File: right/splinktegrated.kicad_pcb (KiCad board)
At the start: 4 copper layers, 72.5 x 88.4 mm, 81 parts, among them J1 USB_C_Receptacle_USB2.0, J10 NA_Ribbon, J13 Conn_01x01_Socket, J14 Cirque, J15 Conn_01x01_Socket, J16 Conn_01x01_Socket, J17 Conn_01x01_Socket, J18 USB_C_Receptacle_USB2.0, J19 Conn_01x01_Socket, J20 Conn_01x01_Socket, J5 Conn_01x02, J6 Cirque, J7 NA_trackball, J8 NA_Ribbon, J9 NA_RGB, Q4 AO3401A, Q5 AO3401A, SW2 NA_SW_SPST, U1 RP2040, U2 USBLC6-2P6, U3 XC6210B332MR-G, U4 USBLC6-2P6, U5 W25Q128JVS, U6 74LVC1T45, Y1 Crystal_GND24

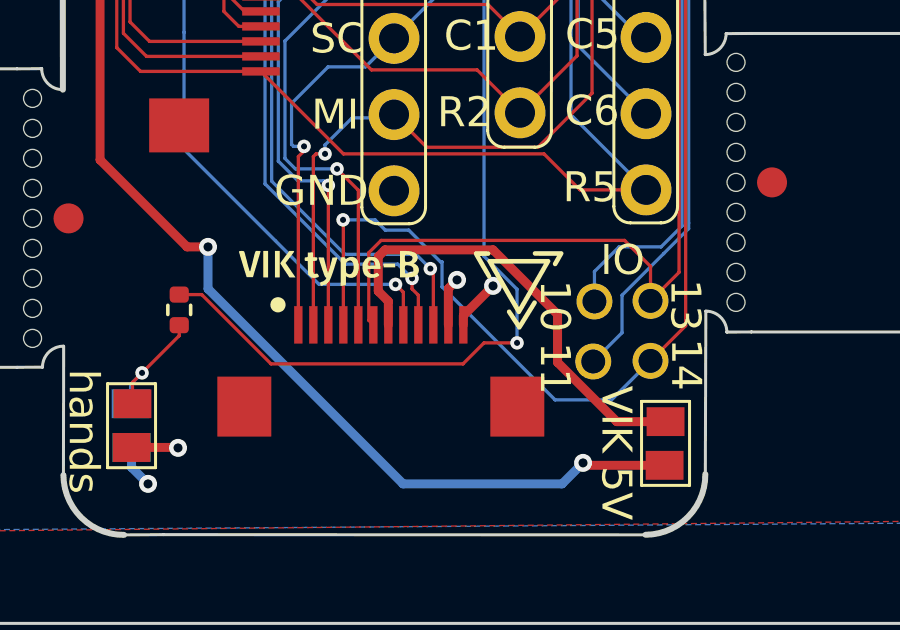
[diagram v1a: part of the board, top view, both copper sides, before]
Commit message: routing
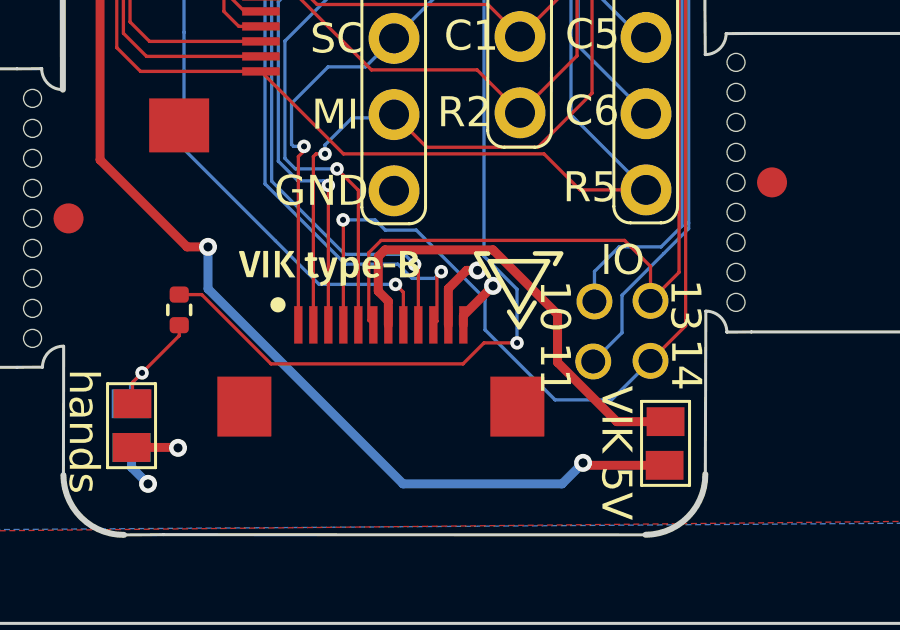
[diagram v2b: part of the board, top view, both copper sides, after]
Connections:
- J6 pad 10: SCL -> SDA
- J6 pad 9: SDA -> SCL
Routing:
- net SDA: track 43.0 -> 44.3 mm
- net GND: track 52.4 -> 53.2 mm
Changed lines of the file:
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@@
 			(size 0.28 1.25)
 			(layers "F.Cu" "F.Mask" "F.Paste")
-			(net 53 "SDA")
+			(net 54 "SCL")
 			(pinfunction "Pin_9")
 			(pintype "passive")
@@
 			(size 0.28 1.25)
 			(layers "F.Cu" "F.Mask" "F.Paste")
-			(net 54 "SCL")
+			(net 53 "SDA")
 			(pinfunction "Pin_10")
 			(pintype "passive")
@@
 	)
 	(segment
+		(start 151.01 129.59)
+		(end 151.01 130.8)
+		(width 0.3)
+		(layer "F.Cu")
+		(net 2)
+	)
+	(segment
 		(start 159.6 88.9)
 		(end 159.35 88.65)
@@
 	)
 	(segment
-		(start 151.01 129.59)
-		(end 151.3 129.3)
-		(width 0.3)
-		(layer "F.Cu")
-		(net 2)
-	)
-	(segment
 		(start 157.96 104.1)
 		(end 158.7 104.1)
@@
 	)
 	(segment
-		(start 151.01 130.8)
+		(start 151.616897 128.983103)
 		(end 151.01 129.59)
 		(width 0.3)
@@
 	)
 	(segment
+		(start 151.984518 128.983103)
+		(end 151.616897 128.983103)
+		(width 0.3)
+		(layer "F.Cu")
+		(net 2)
+	)
+	(segment
 		(start 162.05 99.58)
 		(end 161.9 99.43)
@@
 	)
 	(via
-		(at 151.3 129.3)
+		(at 151.984518 128.983103)
 		(size 0.6)
 		(drill 0.3)
@@
 	)
 	(segment
-		(start 149.8 129.25)
-		(end 149.8 129.6)
+		(start 150.774228 129.025772)
+		(end 150.631 129.169)
 		(width 0.11)
 		(layer "F.Cu")
@@
 	)
 	(segment
-		(start 149.8 129.6)
-		(end 150.01 129.81)
+		(start 150.631 129.169)
+		(end 150.631 130.679)
 		(width 0.11)
 		(layer "F.Cu")
@@
 	)
 	(segment
-		(start 150.01 129.81)
-		(end 150.01 130.8)
+		(start 150.631 130.679)
+		(end 150.51 130.8)
 		(width 0.11)
 		(layer "F.Cu")
@@
 	)
 	(via
-		(at 150.4 97)
+		(at 150.774228 129.025772)
 		(size 0.45)
 		(drill 0.2)
@@
 	)
 	(via
-		(at 149.8 129.25)
+		(at 150.4 97)
 		(size 0.45)
 		(drill 0.2)
@@
 	)
 	(segment
+		(start 149.8 129.25)
+		(end 150.55 129.25)
+		(width 0.11)
+		(layer "B.Cu")
+		(net 53)
+	)
+	(segment
+		(start 150.55 129.25)
+		(end 150.774228 129.025772)
+		(width 0.11)
+		(layer "B.Cu")
+		(net 53)
+	)
+	(segment
 		(start 148.4 103.6)
 		(end 149.3 102.7)
@@
 	)
 	(segment
-		(start 150.51 130.8)
-		(end 150.51 129.025772)
+		(start 150.01 130.8)
+		(end 150.01 128.908458)
 		(width 0.11)
 		(layer "F.Cu")
@@
 	)
 	(segment
-		(start 150.51 129.025772)
-		(end 150.41 128.925772)
+		(start 150.01 128.908458)
+		(end 149.886542 128.785)
 		(width 0.11)
 		(layer "F.Cu")
@@
 	)
 	(via
-		(at 150.41 128.925772)
+		(at 149.886542 128.785)
 		(size 0.45)
 		(drill 0.2)
@@
 	)
 	(segment
-		(start 145.121 115.991541)
-		(end 146.621 114.491542)
+		(start 148.491541 103.821)
+		(end 149.521 102.791542)
 		(width 0.11)
 		(layer "B.Cu")
@@
 	)
 	(segment
-		(start 147.562542 128.45)
-		(end 145.121 126.008458)
+		(start 145.121 115.991541)
+		(end 146.621 114.491542)
 		(width 0.11)
 		(layer "B.Cu")
@@
 	)
 	(segment
-		(start 146.991542 103.821)
-		(end 148.491541 103.821)
+		(start 150.7 97.4)
+		(end 151.1 97)
 		(width 0.11)
 		(layer "B.Cu")
@@
 	)
 	(segment
-		(start 145.121 126.008458)
-		(end 145.121 115.991541)
+		(start 150.7 99.612542)
+		(end 150.7 97.4)
 		(width 0.11)
 		(layer "B.Cu")
@@
 	)
 	(segment
-		(start 150.7 99.612542)
-		(end 150.7 97.4)
+		(start 146.621 104.191542)
+		(end 146.991542 103.821)
 		(width 0.11)
 		(layer "B.Cu")
@@
 	)
 	(segment
-		(start 148.491541 103.821)
-		(end 149.521 102.791542)
+		(start 145.121 126.008458)
+		(end 145.121 115.991541)
 		(width 0.11)
 		(layer "B.Cu")
@@
 	)
 	(segment
-		(start 146.621 104.191542)
-		(end 146.991542 103.821)
+		(start 146.991542 103.821)
+		(end 148.491541 103.821)
 		(width 0.11)
 		(layer "B.Cu")
@@
 	)
 	(segment
-		(start 149.934228 128.45)
+		(start 149.551542 128.45)
 		(end 147.562542 128.45)
 		(width 0.11)
@@
 	)
 	(segment
-		(start 149.521 102.791542)
-		(end 149.521 100.791542)
+		(start 149.521 100.791542)
+		(end 150.7 99.612542)
 		(width 0.11)
 		(layer "B.Cu")
@@
 	)
 	(segment
-		(start 150.41 128.925772)
-		(end 149.934228 128.45)
+		(start 149.521 102.791542)
+		(end 149.521 100.791542)
 		(width 0.11)
 		(layer "B.Cu")
@@
 	)
 	(segment
-		(start 149.521 100.791542)
-		(end 150.7 99.612542)
+		(start 146.621 114.491542)
+		(end 146.621 104.191542)
 		(width 0.11)
 		(layer "B.Cu")
@@
 	)
 	(segment
-		(start 146.621 114.491542)
-		(end 146.621 104.191542)
+		(start 147.562542 128.45)
+		(end 145.121 126.008458)
 		(width 0.11)
 		(layer "B.Cu")
@@
 	)
 	(segment
-		(start 150.7 97.4)
-		(end 151.1 97)
+		(start 149.886542 128.785)
+		(end 149.551542 128.45)
 		(width 0.11)
 		(layer "B.Cu")
@@
 	)
 	(segment
-		(start 150.75 128.7)
-		(end 149.690948 127.640948)
+		(start 148.909052 127.640948)
+		(end 148.568105 127.3)
 		(width 0.11)
 		(layer "B.Cu")
@@
 	)
 	(segment
-		(start 148.568105 127.3)
-		(end 147.5 127.3)
+		(start 157.75 132)
+		(end 156.45 133.3)
 		(width 0.11)
 		(layer "B.Cu")
@@
 	)
 	(segment
-		(start 155.416458 107.983542)
-		(end 155.416458 106.671)
+		(start 149.940948 127.640948)
+		(end 148.909052 127.640948)
 		(width 0.11)
 		(layer "B.Cu")
@@
 	)
 	(segment
-		(start 148.909052 127.640948)
-		(end 148.568105 127.3)
+		(start 154.568105 133.3)
+		(end 152.234052 130.965948)
 		(width 0.11)
 		(layer "B.Cu")
@@
 	)
 	(segment
-		(start 154.836362 109.663638)
-		(end 156.1 108.4)
+		(start 155.416458 107.983542)
+		(end 155.416458 106.671)
 		(width 0.11)
 		(layer "B.Cu")
@@
 	)
 	(segment
-		(start 159 110.8)
-		(end 158.687458 110.8)
+		(start 152.234052 129.934052)
+		(end 149.940948 127.640948)
 		(width 0.11)
 		(layer "B.Cu")
@@
 	)
 	(segment
-		(start 155.149541 103.429)
-		(end 154.779 103.429)
+		(start 154.836362 109.663638)
+		(end 156.1 108.4)
 		(width 0.11)
 		(layer "B.Cu")
@@
 	)
 	(segment
-		(start 154.836362 110.488579)
-		(end 154.836362 109.663638)
+		(start 159 110.8)
+		(end 158.687458 110.8)
 		(width 0.11)
 		(layer "B.Cu")
@@
 	)
 	(segment
-		(start 157.75 132)
-		(end 156.45 133.3)
+		(start 155.149541 103.429)
+		(end 154.779 103.429)
 		(width 0.11)
 		(layer "B.Cu")
@@
 	)
 	(segment
-		(start 149.690948 127.640948)
-		(end 148.909052 127.640948)
+		(start 154.836362 110.488579)
+		(end 154.836362 109.663638)
 		(width 0.11)
 		(layer "B.Cu")
@@
 	)
 	(segment
-		(start 156.45 133.3)
-		(end 154.568105 133.3)
+		(start 148.568105 127.3)
+		(end 147.5 127.3)
 		(width 0.11)
 		(layer "B.Cu")
@@
 	)
 	(segment
-		(start 150.8 128.7)
-		(end 150.75 128.7)
+		(start 156.097783 111.75)
+		(end 154.836362 110.488579)
 		(width 0.11)
 		(layer "B.Cu")
@@
 	)
 	(segment
-		(start 156.097783 111.75)
-		(end 154.836362 110.488579)
+		(start 156.45 133.3)
+		(end 154.568105 133.3)
 		(width 0.11)
 		(layer "B.Cu")
@@
 	)
 	(segment
-		(start 154.568105 133.3)
-		(end 150.8 129.531896)
+		(start 152.234052 130.965948)
+		(end 152.234052 129.934052)
 		(width 0.11)
 		(layer "B.Cu")
@@
 		(width 0.11)
 		(layer "B.Cu")
-		(net 58)
-	)
-	(segment
-		(start 150.8 129.531896)
-		(end 150.8 128.7)
-		(width 0.11)
-		(layer "B.Cu")
